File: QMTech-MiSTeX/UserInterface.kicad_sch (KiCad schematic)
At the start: 38 parts, among them CN2 U.FL-R-SMT-1(80), CN3 U.FL-R-SMT-1(80), CN4 U.FL-R-SMT-1(80), SW1 TS-1187A-B-A-B, SW2 TS-1187A-B-A-B, SW3 TS-1187A-B-A-B, SW4 TS-1187A-B-A-B, U6 HX 0.5-24P XGXJ-H2.0

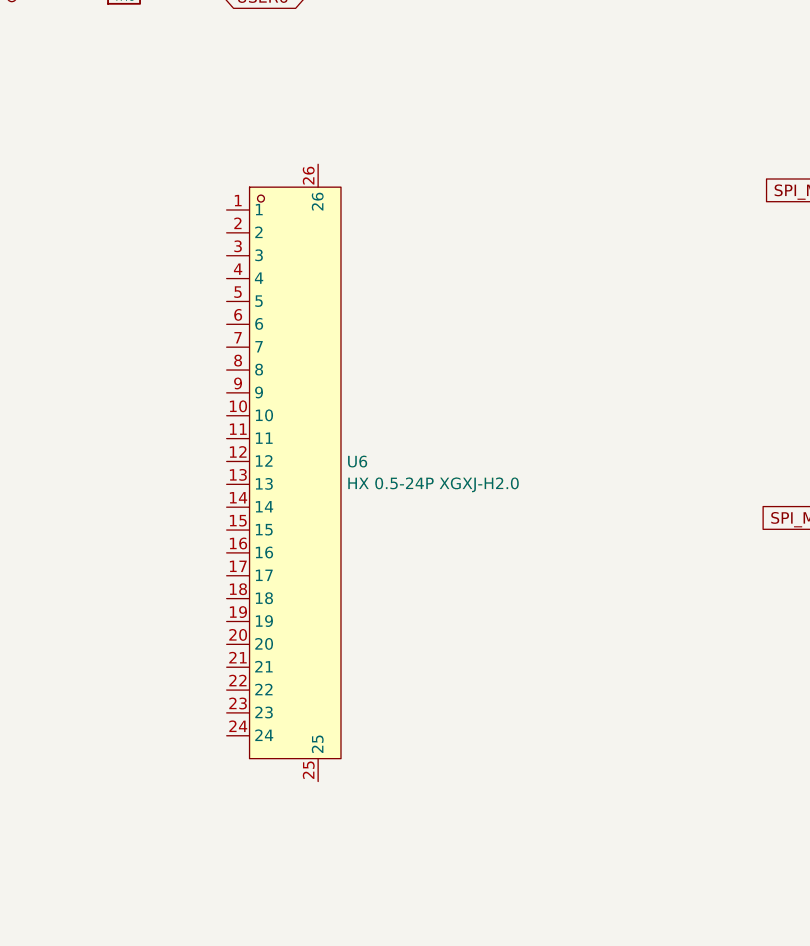
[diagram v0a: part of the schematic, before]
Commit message: QMTech-MiSTeX WIP
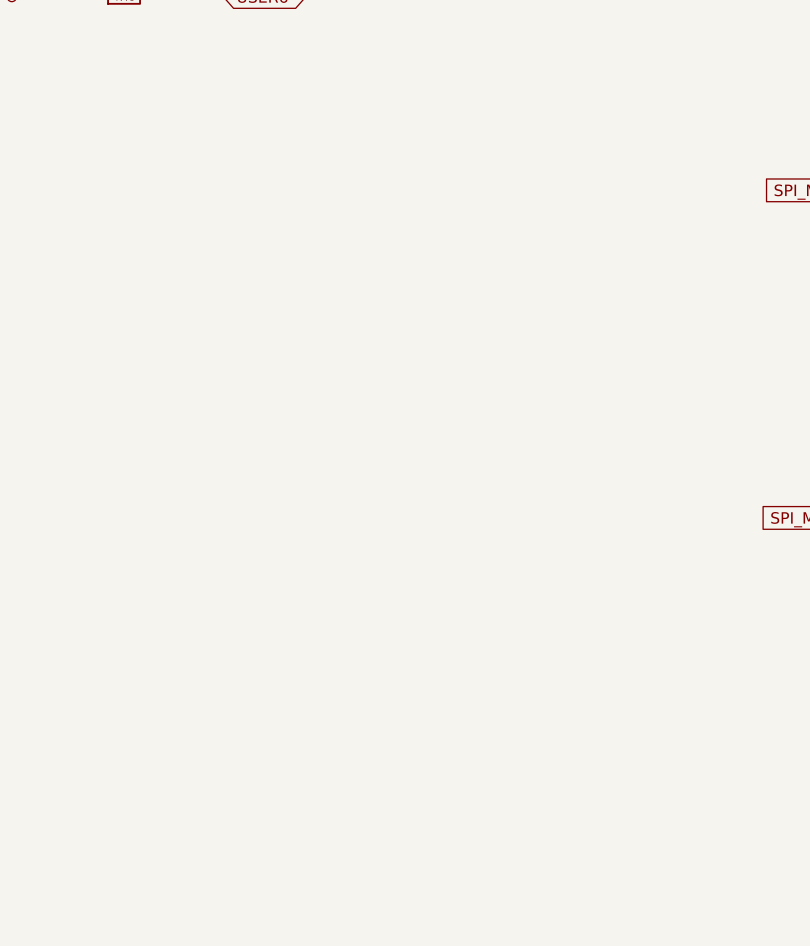
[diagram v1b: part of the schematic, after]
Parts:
- removed U6: HX 0.5-24P XGXJ-H2.0, easyeda2kicad:CONN-SMD_24P-P0.50_HANXIA_HX0.5-24PXGXJ-H2.0, symbol easyeda2kicad:HX0.5-24PXGXJ-H2.0
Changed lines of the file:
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@@
-    )
-  )
-  (symbol (lib_id "easyeda2kicad:HX0.5-24PXGXJ-H2.0") (at 148.2598 107.5182 0) (unit 1)
-    (in_bom yes) (on_board yes) (dnp no) (fields_autoplaced)
-    (property "Reference" "U6" (at 156.5148 105.0361 0)
-      (effects (font (size 1.27 1.27)) (justify left))
-    )
-    (property "Value" "HX 0.5-24P XGXJ-H2.0" (at 156.5148 107.4603 0)
-      (effects (font (size 1.27 1.27)) (justify left))
-    )
-    (property "Footprint" "easyeda2kicad:CONN-SMD_24P-P0.50_HANXIA_HX0.5-24PXGXJ-H2.0" (at 148.2598 148.1582 0)
-      (effects (font (size 1.27 1.27)) hide)
-    )
-    (property "Datasheet" "" (at 148.2598 107.5182 0)
-      (effects (font (size 1.27 1.27)) hide)
-    )
-    (property "LCSC Part" "C5142050" (at 148.2598 150.6982 0)
-      (effects (font (size 1.27 1.27)) hide)
-    )
-    (pin "3")
-    (pin "26")
-    (pin "24")
-    (pin "8")
-    (pin "4")
-    (pin "7")
-    (pin "15")
-    (pin "14")
-    (pin "12")
-    (pin "13")
-    (pin "11")
-    (pin "6")
-    (pin "19")
-    (pin "9")
-    (pin "1")
-    (pin "10")
-    (pin "2")
-    (pin "22")
-    (pin "16")
-    (pin "21")
-    (pin "18")
-    (pin "20")
-    (pin "5")
-    (pin "23")
-    (pin "17")
-    (pin "25")
-    (instances
-      (project "QMTech-MiSTeX"
-        (path "/bf95850e-2fcb-4784-a603-f17fc357556b/cce2b405-ae09-44af-ba42-d113d6ffe521"
-          (reference "U6") (unit 1)
-        )
-      )
     )
   )
